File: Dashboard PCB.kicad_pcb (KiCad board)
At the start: 2 copper layers, 130 x 100.2 mm, 62 parts, among them J1 Controls_Leader_Export_02x06, J2 Conn_02x03_CAN, J3 INDICATOR_SWITCH_OUT, J4 FAN_CTRL_01x02, J5 Horn_In_01x02, J6 Horn_Out_01x02, J7 Conn_02x03_CAN

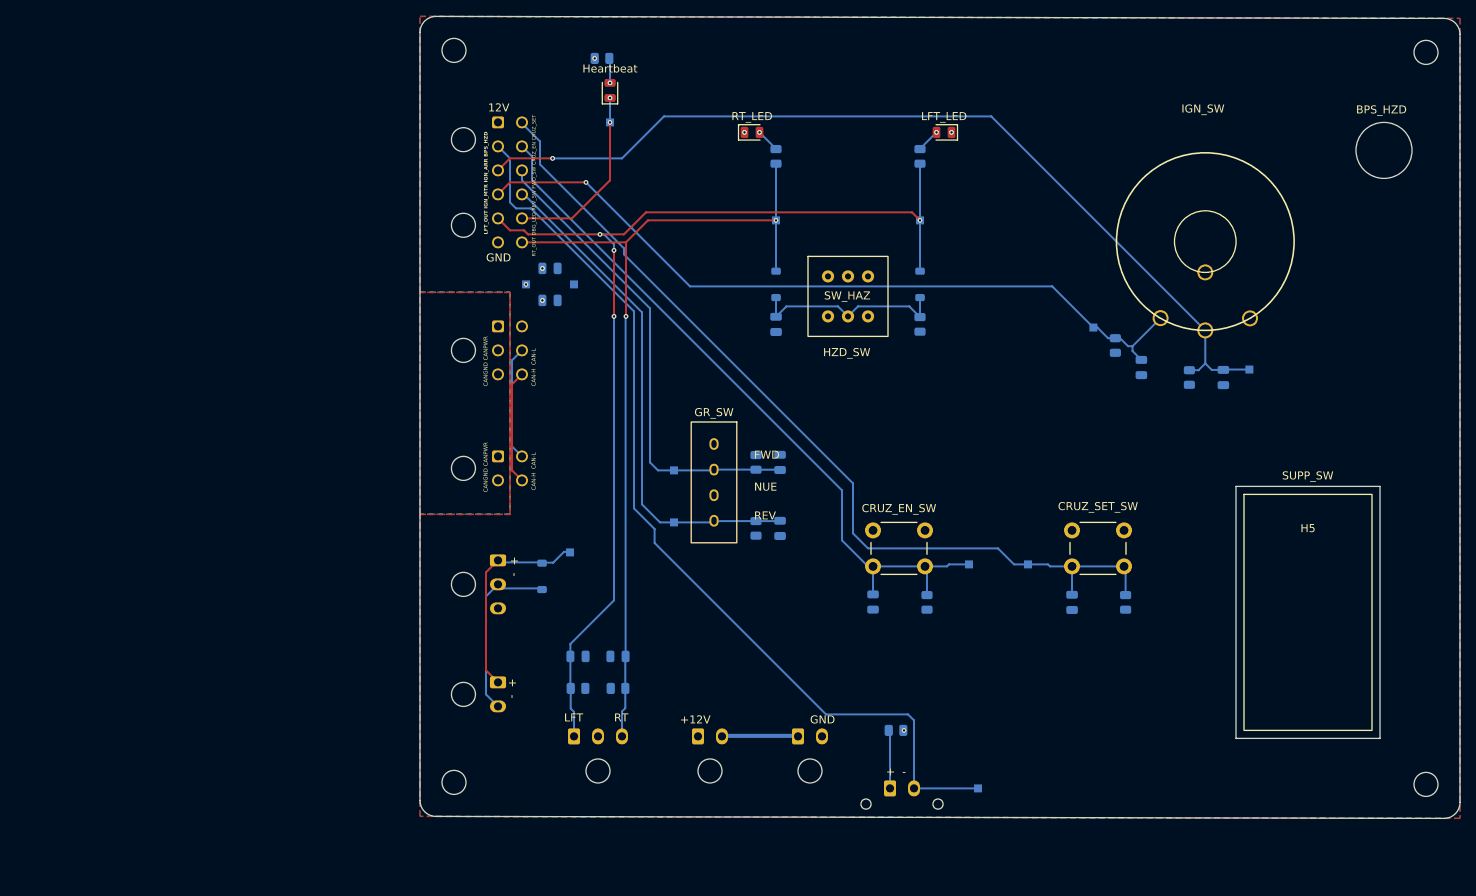
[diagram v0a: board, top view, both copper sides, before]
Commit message: A bunch of stuff
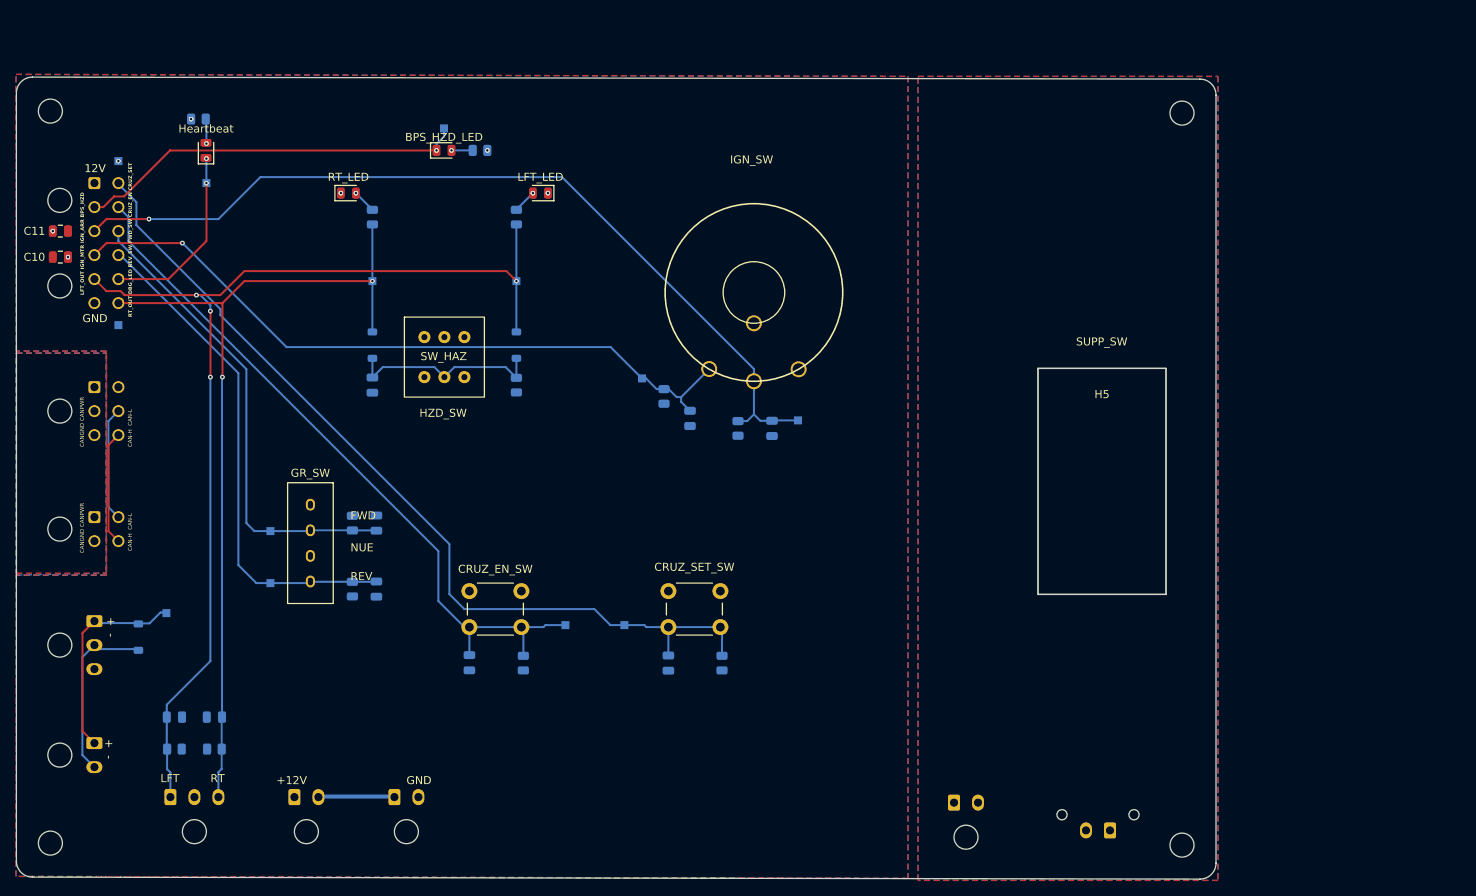
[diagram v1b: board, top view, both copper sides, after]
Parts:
- removed BPS_HZD_OUT: BPS_HAZARD_LIGHT, Connector_Molex:Molex_Micro-Fit_3.0_43650-0215_1x02_P3.00mm_Vertical
- added BPS_HZD_LED: SMD_0805_RED, LED_SMD:LED_0805_2012Metric, F.Cu at (137.0, 59.5)
- added J8: Supp_Out, Connector_Molex:Molex_Micro-Fit_3.0_43650-0200_1x02_P3.00mm_Horizontal, B.Cu at (200.8, 141.0)
- added Supp Sw Connectors: Supp_In, Connector_Molex:Molex_Micro-Fit_3.0_43650-0215_1x02_P3.00mm_Vertical, B.Cu at (220.2, 144.5)
- C10, C11: moved to F.Cu
- moved BPS_HZD 106.1 mm to (137.0, 56.8)
- moved R13 89.2 mm to (141.5, 59.5)
- moved C11 61.8 mm to (89.0, 69.6), turned to 180 degrees
- moved C10 61.2 mm to (89.0, 72.8)
- moved GND 57.2 mm to (96.3, 81.3)
- moved C5 56.8 mm to (178.0, 94.2)
- moved C6 56.8 mm to (167.8, 93.0)
- moved IGN_ARR 56.8 mm to (181.2, 93.2)
- moved IGN_MTR 56.8 mm to (161.8, 88.0)
- moved IGN_SW1 56.8 mm to (175.8, 77.2)
- moved R5 56.8 mm to (173.8, 94.2)
- moved R6 56.8 mm to (164.5, 90.2)
- moved +12V 53.2 mm to (96.3, 60.8)
- moved Heartbeat 51.1 mm to (107.2, 59.5)
- moved C1 51.0 mm to (103.3, 130.3)
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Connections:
- net /IGN_PWR renamed /IGN_MTR
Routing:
- net /BPS_HZD: track 116.9 -> 48.8 mm, vias 0 -> 1
- net /IGN_MTR: track 95.5 -> 89.1 mm
- net /IGN_ARR: track 114.8 -> 109.2 mm
- net Net-(BPS_HZD_LED1-A): track 7.28 -> 3.00 mm, vias 0 -> 1
- net GND: vias 2 -> 4
- net +12V: vias 5 -> 3
- added copper zone on F.Cu, net /Supp+
- added copper zone on B.Cu, net /Supp-
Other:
- board size 130 x 100.2 mm -> 150 x 100.2 mm
- board text added: "- +"
- board text removed: "Approx 3d model"
- board text removed: "BPS_HZD"
- board text removed: "Mounting pt for BPS led (Still need dimensions)"
